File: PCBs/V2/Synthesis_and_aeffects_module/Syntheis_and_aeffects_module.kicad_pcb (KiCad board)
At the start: 2 copper layers, 83.5 x 60 mm, 27 parts, among them J1 AudioJack3_SwitchTR, J2 IN, J3 OUT, U1 STM32H750VBTx, U2 TPA6110A2DGN

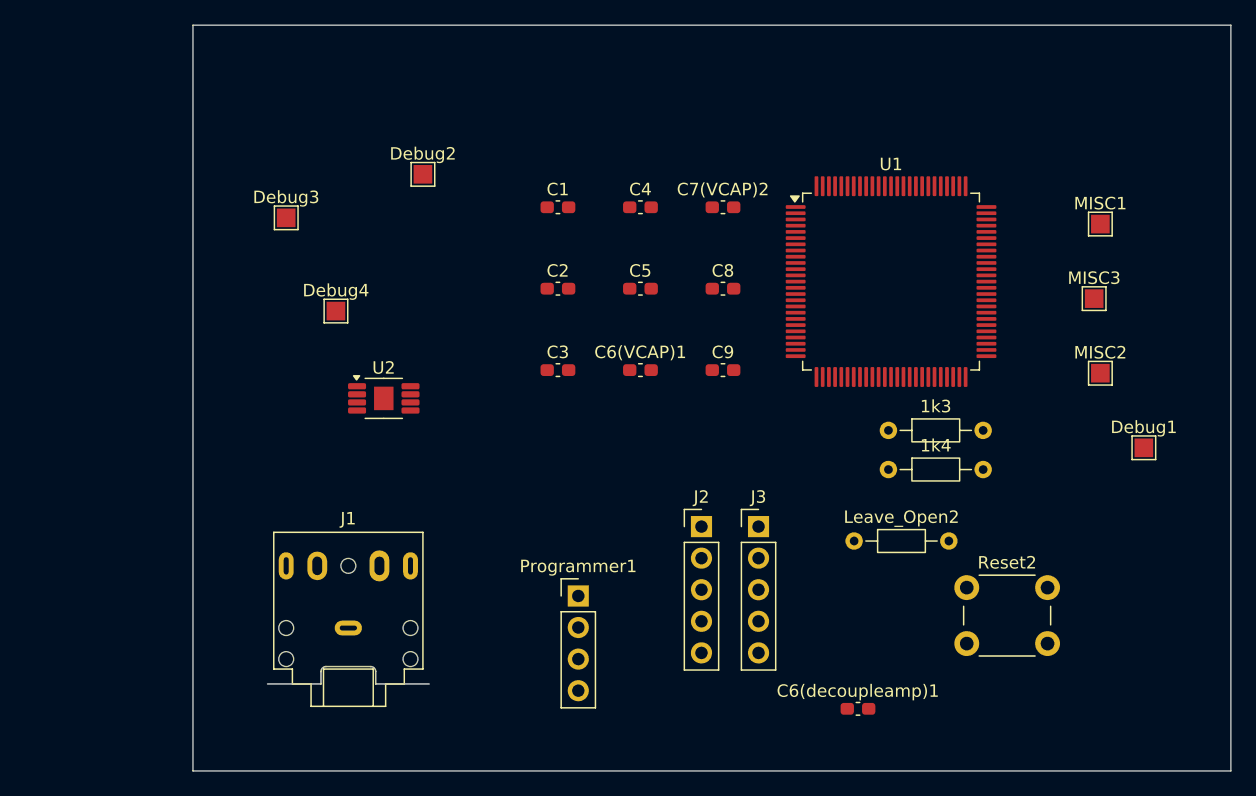
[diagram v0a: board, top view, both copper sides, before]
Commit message: schematic progress
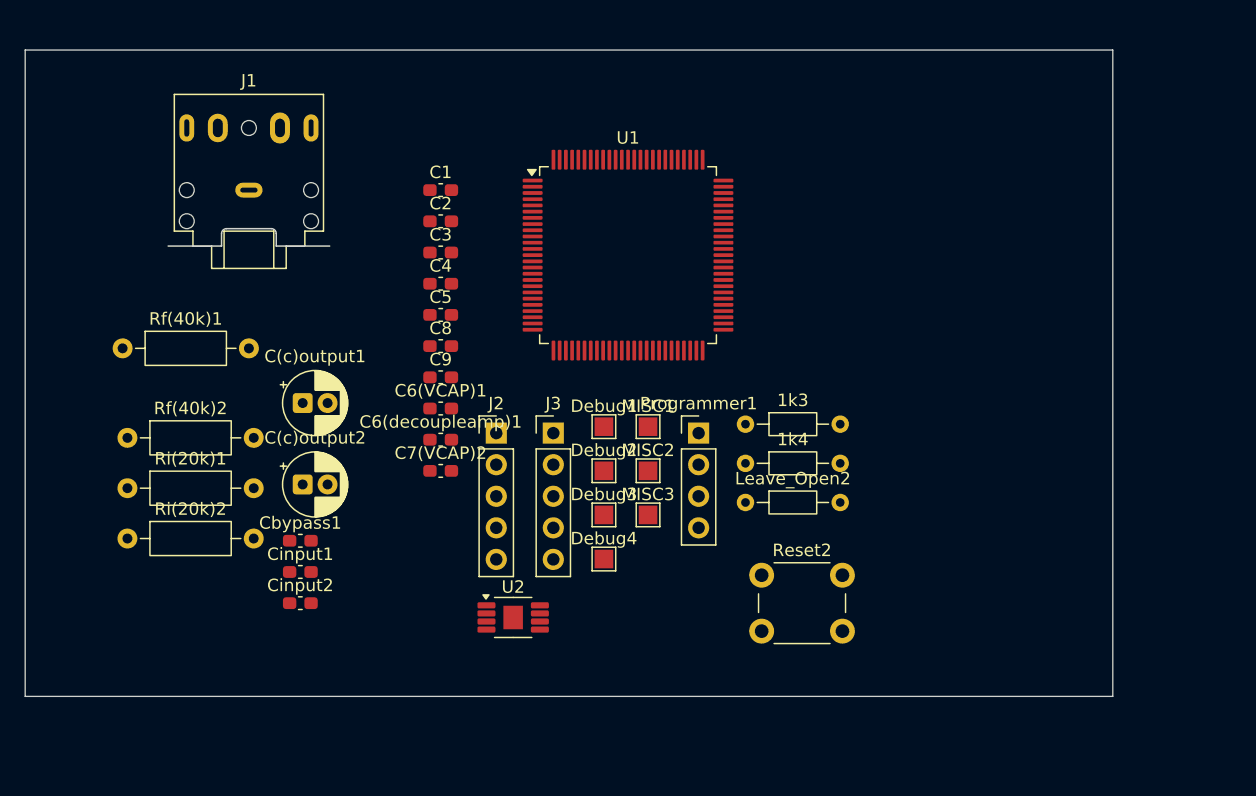
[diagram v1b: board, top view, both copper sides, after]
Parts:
- added C(c)output1: 220uf, Capacitor_THT:CP_Radial_D5.0mm_P2.00mm, F.Cu at (83.8, 89.4)
- added C(c)output2: 220uf, Capacitor_THT:CP_Radial_D5.0mm_P2.00mm, F.Cu at (83.8, 96.0)
- added Cbypass1: 0.47uf(LOW ESR), Capacitor_SMD:C_0603_1608Metric_Pad1.08x0.95mm_HandSolder, F.Cu at (83.6, 100.5)
- added Cinput1: 0.47uf, Capacitor_SMD:C_0603_1608Metric_Pad1.08x0.95mm_HandSolder, F.Cu at (83.6, 103.0)
- added Cinput2: 0.47uf, Capacitor_SMD:C_0603_1608Metric_Pad1.08x0.95mm_HandSolder, F.Cu at (83.6, 105.5)
- added Rf(40k)1: 40k, Resistor_THT:R_Axial_DIN0207_L6.3mm_D2.5mm_P10.16mm_Horizontal, F.Cu at (69.3, 85.0)
- added Rf(40k)2: 40k, Resistor_THT:R_Axial_DIN0207_L6.3mm_D2.5mm_P10.16mm_Horizontal, F.Cu at (69.7, 92.2)
- added Ri(20k)1: 20k, Resistor_THT:R_Axial_DIN0207_L6.3mm_D2.5mm_P10.16mm_Horizontal, F.Cu at (69.7, 96.2)
- added Ri(20k)2: 20k, Resistor_THT:R_Axial_DIN0207_L6.3mm_D2.5mm_P10.16mm_Horizontal, F.Cu at (69.7, 100.3)
- moved Debug1 43.5 mm to (108.1, 91.3)
- moved C6(decoupleamp)1 39.9 mm to (94.9, 92.3)
- moved MISC3 39.9 mm to (111.6, 98.4)
- moved MISC1 39.9 mm to (111.6, 91.3)
- moved MISC2 37.2 mm to (111.6, 94.8)
- moved J1 36.1 mm to (79.5, 72.3)
- moved Debug3 35.0 mm to (108.1, 98.4)
- moved C7(VCAP)2 31.1 mm to (94.9, 94.9)
- moved Debug4 29.4 mm to (108.1, 102.0)
- moved Debug2 27.9 mm to (108.1, 94.8)
- moved C8 23.2 mm to (94.9, 84.8)
- moved C9 22.7 mm to (94.9, 87.3)
- moved U1 21.3 mm to (110.0, 77.5)
- moved U2 20.5 mm to (100.8, 106.7)
- moved J3 18.1 mm to (104.0, 91.8)
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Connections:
- C6(decoupleamp)1 pad 1: unconnected-(C6(decoupleamp)1-Pad1) -> /VCC
- C6(decoupleamp)1 pad 2: unconnected-(C6(decoupleamp)1-Pad2) -> Net-(U2-VDD)
- J1 pad R: unconnected-(J1-PadR) -> Net-(C(c)output2-Pad2)
- U2 pad 3: GNDPWR -> /VCC
- U2 pad 4: Net-(U2-IN2-) -> Net-(U2-IN1-)
- U2 pad 6: /VCC -> Net-(U2-VDD)
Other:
- board size 83.5 x 60 mm -> 87.5 x 52 mm
